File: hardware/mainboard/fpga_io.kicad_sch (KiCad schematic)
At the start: 24 parts, among them U1 LIFCL_40_CABGA400, X1 XO32

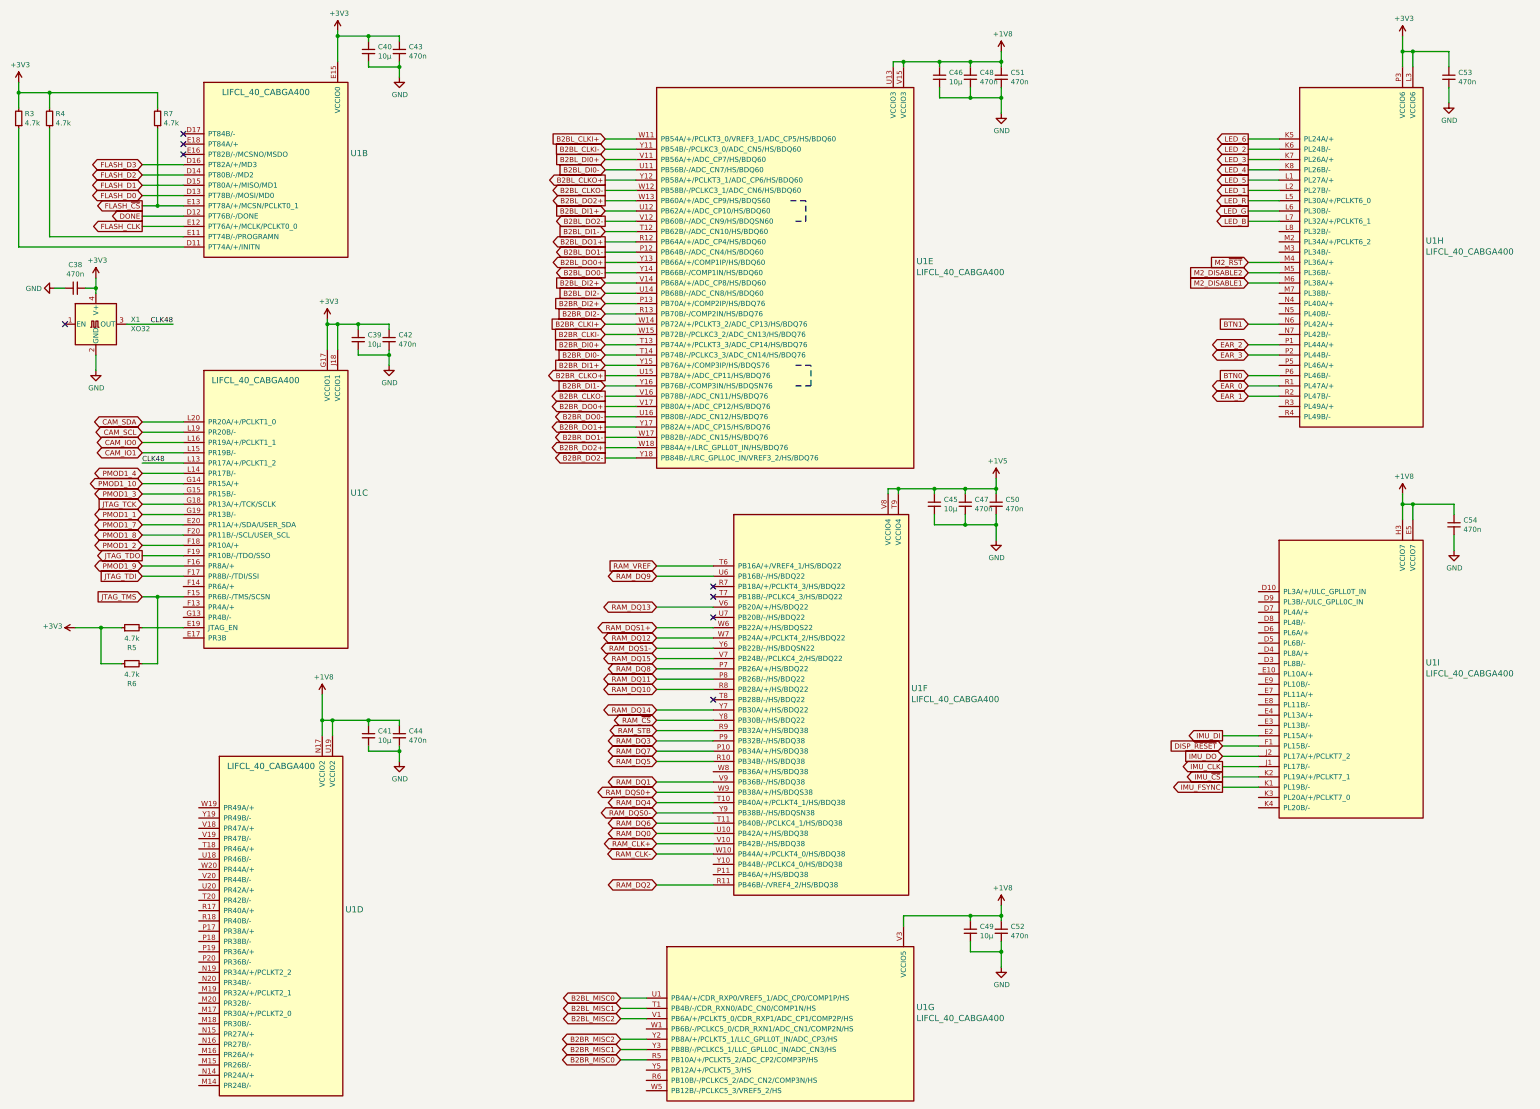
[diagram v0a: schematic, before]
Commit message: First pass at routing done
Signed-off-by: David Shah <dave@ds0.me>
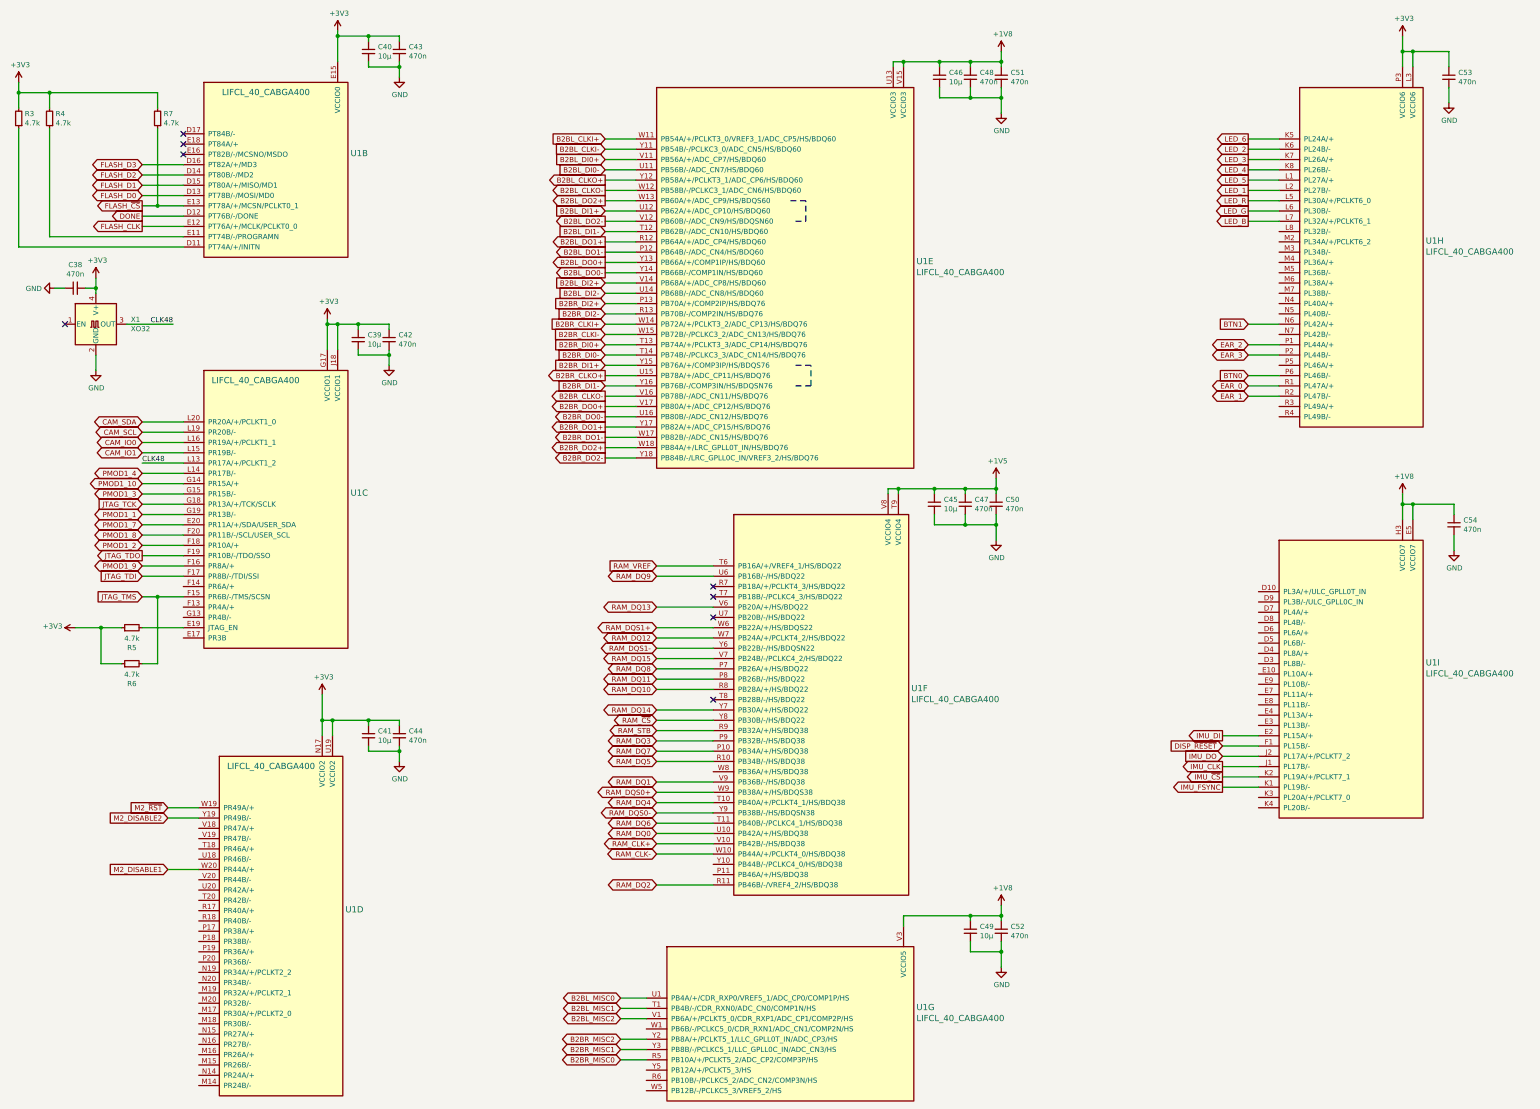
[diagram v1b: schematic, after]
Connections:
- net +1V8: no longer C41.1, C44.1, U1.N17 (VCCIO2), U1.U19 (VCCIO2)
- net +3V3: now also C41.1, C44.1, U1.N17 (VCCIO2), U1.U19 (VCCIO2)
- net M2_DISABLE1: now also U1.W20 (PR44A/+); no longer U1.M6 (PL38A/+)
- net M2_DISABLE2: now also U1.Y19 (PR49B/-); no longer U1.M5 (PL36B/-)
- net M2_~RST: now also U1.W19 (PR49A/+); no longer U1.M4 (PL36A/+)
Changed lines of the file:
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@@
+    (stroke (width 0) (type solid) (color 0 0 0 0))
+  )
+  (wire (pts (xy 57.15 210.82) (xy 64.77 210.82))
+    (stroke (width 0) (type solid) (color 0 0 0 0))
+  )
+  (wire (pts (xy 57.15 213.36) (xy 64.77 213.36))
+    (stroke (width 0) (type solid) (color 0 0 0 0))
+  )
+  (wire (pts (xy 57.15 226.06) (xy 64.77 226.06))
     (stroke (width 0) (type solid) (color 0 0 0 0))
   )
@@
   )
   (wire (pts (xy 323.85 66.04) (xy 331.47 66.04))
-    (stroke (width 0) (type solid) (color 0 0 0 0))
-  )
-  (wire (pts (xy 323.85 76.2) (xy 331.47 76.2))
-    (stroke (width 0) (type solid) (color 0 0 0 0))
-  )
-  (wire (pts (xy 323.85 78.74) (xy 331.47 78.74))
-    (stroke (width 0) (type solid) (color 0 0 0 0))
-  )
-  (wire (pts (xy 323.85 81.28) (xy 331.47 81.28))
     (stroke (width 0) (type solid) (color 0 0 0 0))
   )
@@
     )
   )
+  (global_label "M2_~RST" (shape input) (at 57.15 210.82 180)
+    (effects (font (size 1.27 1.27)) (justify right))
+    (property "Intersheet References" "${INTERSHEET_REFS}" (id 0) (at 52.9228 210.7406 0)
+      (effects (font (size 1.27 1.27)) (justify left) hide)
+    )
+  )
+  (global_label "M2_DISABLE2" (shape input) (at 57.15 213.36 180)
+    (effects (font (size 1.27 1.27)) (justify right))
+    (property "Intersheet References" "${INTERSHEET_REFS}" (id 0) (at 58.3052 213.2806 0)
+      (effects (font (size 1.27 1.27)) (justify left) hide)
+    )
+  )
+  (global_label "M2_DISABLE1" (shape input) (at 57.15 226.06 180)
+    (effects (font (size 1.27 1.27)) (justify right))
+    (property "Intersheet References" "${INTERSHEET_REFS}" (id 0) (at 58.3052 225.9806 0)
+      (effects (font (size 1.27 1.27)) (justify left) hide)
+    )
+  )
   (global_label "B2BL_CLKI+" (shape input) (at 165.1 45.72 180)
     (effects (font (size 1.27 1.27)) (justify right))
@@
     (property "Intersheet References" "${INTERSHEET_REFS}" (id 0) (at 314.2281 65.9606 0)
       (effects (font (size 1.27 1.27)) (justify right) hide)
-    )
-  )
-  (global_label "M2_~RST" (shape input) (at 323.85 76.2 180)
-    (effects (font (size 1.27 1.27)) (justify right))
-    (property "Intersheet References" "${INTERSHEET_REFS}" (id 0) (at 319.6228 76.1206 0)
-      (effects (font (size 1.27 1.27)) (justify left) hide)
-    )
-  )
-  (global_label "M2_DISABLE2" (shape input) (at 323.85 78.74 180)
-    (effects (font (size 1.27 1.27)) (justify right))
-    (property "Intersheet References" "${INTERSHEET_REFS}" (id 0) (at 325.0052 78.6606 0)
-      (effects (font (size 1.27 1.27)) (justify left) hide)
-    )
-  )
-  (global_label "M2_DISABLE1" (shape input) (at 323.85 81.28 180)
-    (effects (font (size 1.27 1.27)) (justify right))
-    (property "Intersheet References" "${INTERSHEET_REFS}" (id 0) (at 325.0052 81.2006 0)
-      (effects (font (size 1.27 1.27)) (justify left) hide)
     )
   )
@@
     (pin "1")
   )
-  (symbol (lib_id "power:+1V8") (at 95.25 182.88 0) (unit 1)
+  (symbol (lib_id "power:+3V3") (at 95.25 182.88 0) (unit 1)
     (in_bom yes) (on_board yes)
-    (property "Reference" "#PWR032" (id 0) (at 95.25 186.69 0)
+    (property "Reference" "#PWR0114" (id 0) (at 95.25 186.69 0)
       (effects (font (size 1.27 1.27)) hide)
     )
-    (property "Value" "+1V8" (id 1) (at 95.6183 178.5556 0))
+    (property "Value" "+3V3" (id 1) (at 95.6183 178.5556 0))
     (property "Footprint" "" (id 2) (at 95.25 182.88 0)
       (effects (font (size 1.27 1.27)) hide)
